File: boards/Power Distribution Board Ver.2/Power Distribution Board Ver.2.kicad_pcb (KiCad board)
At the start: 4 copper layers, 127 x 127 mm, 93 parts, among them J1 Screw_Terminal_01x02, J2 Screw_Terminal_01x06, J3 Screw_Terminal_01x06, J4 Screw_Terminal_01x06, K1 Relay, K2 Relay, K3 Relay, K4 Relay, K5 Relay, K6 Relay, SW1 SW_Push_Open, U1 SIC431AED-T1-GE3, U2 SIC431AED-T1-GE3, U3 SIC431AED-T1-GE3

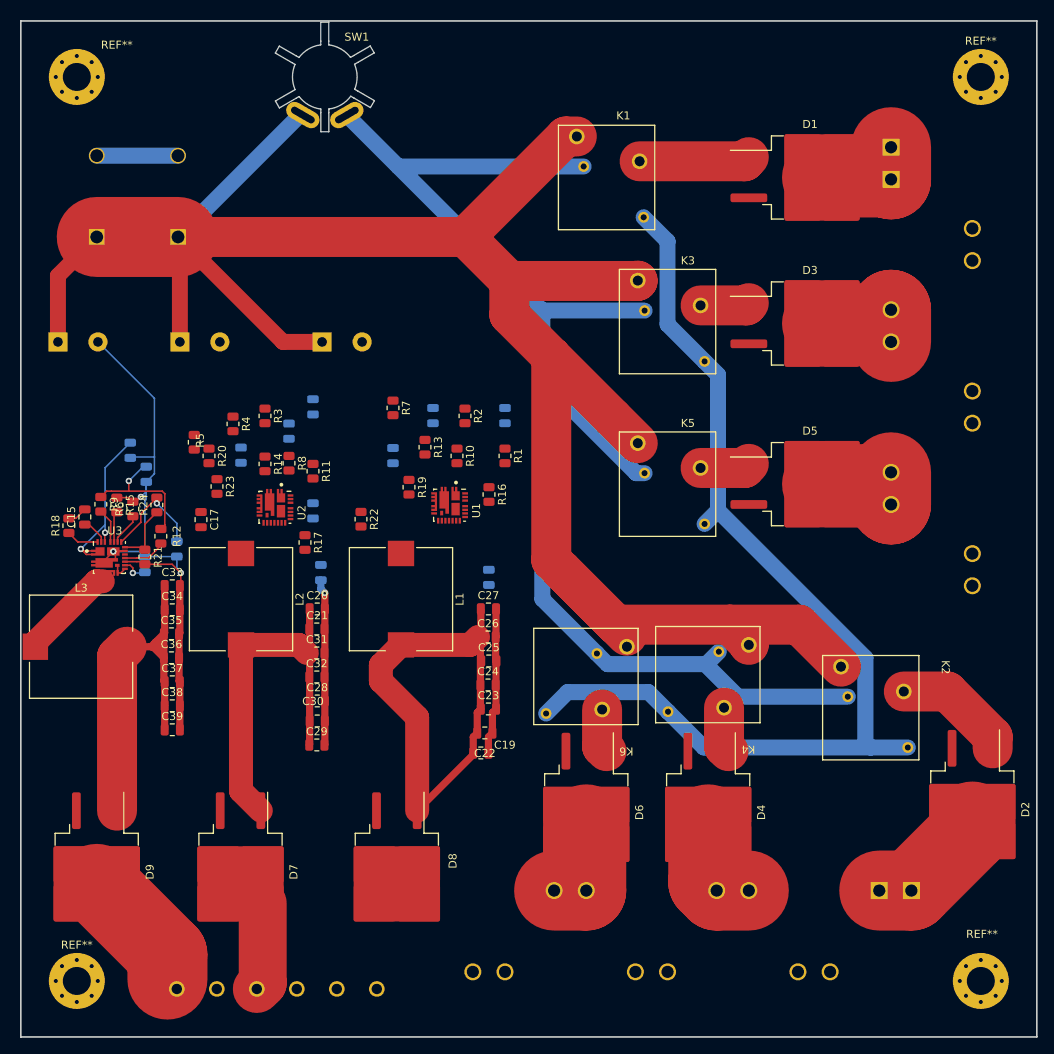
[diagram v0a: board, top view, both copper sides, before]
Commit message: Design Mostly Done
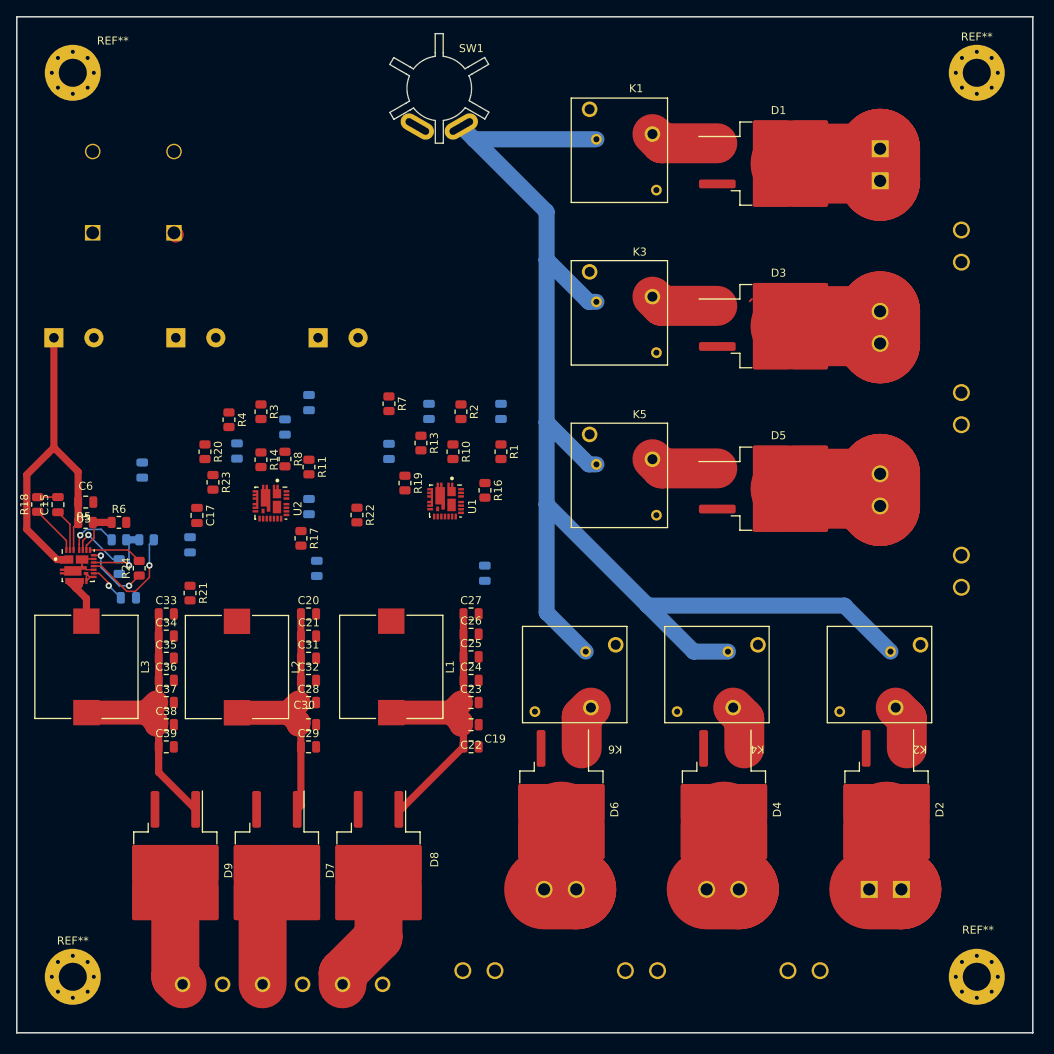
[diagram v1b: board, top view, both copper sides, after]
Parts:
- C6: moved to F.Cu
- R12, R15, R9: moved to B.Cu
- moved R5 16.9 mm to (44.1, 93.7), turned to 0 degrees
- moved SW1 14.4 mm to (88.3, 39.4)
- moved D2 10.7 mm to (144.2, 129.6)
- moved D9 9.83 mm to (55.3, 137.2)
- moved L1 8.55 mm to (82.3, 111.7)
- moved C6 8.54 mm to (44.1, 91.1), turned to 0 degrees
- moved L2 8.49 mm to (63.0, 111.8)
- moved R24 8.21 mm to (50.8, 99.4)
- moved R15 7.71 mm to (48.3, 99.2), turned to 90 degrees
- moved R21 7.23 mm to (57.1, 102.5)
- moved K3 6.12 mm to (115.0, 62.4)
- moved K5 6.12 mm to (115.0, 82.7)
- moved K2 5.53 mm to (148.5, 116.8), turned to 180 degrees
- moved R9 4.98 mm to (48.3, 95.8), turned to 180 degrees
- moved R18 4.71 mm to (38.1, 91.4)
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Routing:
- net GND: track 261.4 -> 3.92 mm, vias 4 -> 0
- net /V_BAT_IN: track 294.7 -> 47.2 mm, vias 2 -> 0
- net Net-(D8-A): track 62.2 -> 39.2 mm
- net Net-(D9-A): track 62.6 -> 44.4 mm, vias 1 -> 0
- net /5V_OUT_3: track 0.00 -> 14.6 mm
- net Net-(D7-A): track 47.4 -> 34.9 mm
- net Net-(D2-A): track 14.9 -> 5.68 mm
- net Net-(U3-PGOOD): track 5.39 -> 13.9 mm, vias 0 -> 1
- net Net-(U3-VDD): track 17.2 -> 9.56 mm
- net /12V_IN_1: track 12.7 -> 18.9 mm
- net /12V_IN_2: track 13.4 -> 19.3 mm
- net Net-(D1-A): track 13.9 -> 8.59 mm
- net /12V_IN_3: track 13.7 -> 18.9 mm
- net Net-(L3-Pad1): track 12.1 -> 7.79 mm
- net Net-(U3-MODE2): track 3.86 -> 7.28 mm, vias 0 -> 1
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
